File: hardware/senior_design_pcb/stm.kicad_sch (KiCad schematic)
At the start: 46 parts, among them J1 SBH11-PBPC-D05-ST-BK, J2 USB_C_Receptacle_USB2.0_16P, J3 Conn_01x03_Socket, J4 Conn_02x08_Odd_Even, J5 Conn_01x03_Socket, J6 Conn_01x03_Socket, SW1 SW_Push, U1 LD1117S33TR_SOT223, U2 STM32F091RCTx, U3 FT232RL, X1 32.768kHz(12.5pF), X3 8MHz(20pF)

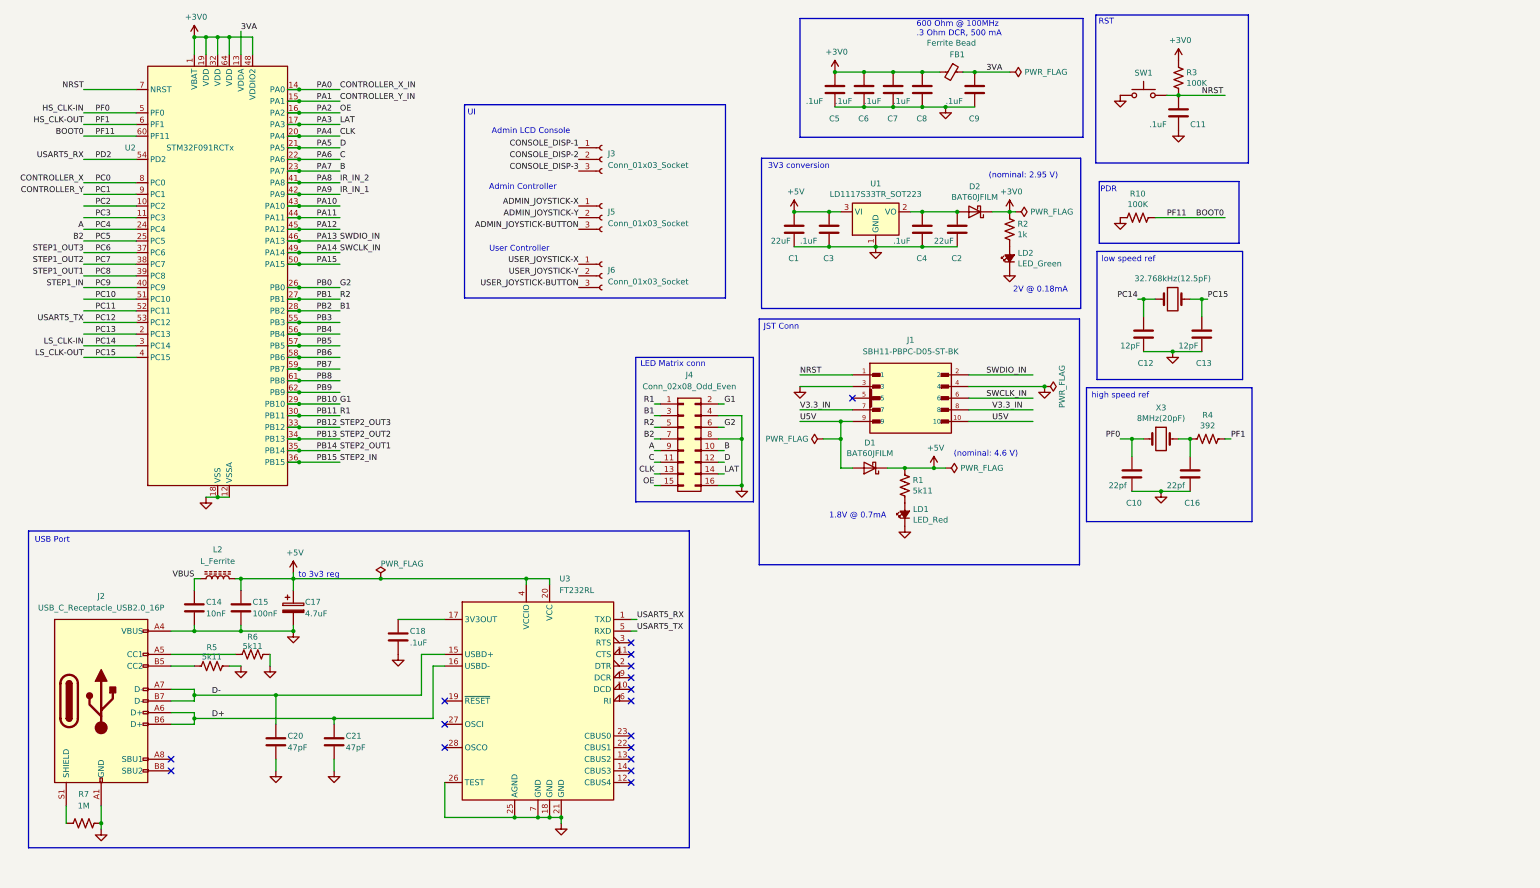
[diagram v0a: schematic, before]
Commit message: small tweaks
added connectors
added shapes
added button
moved shapes
made bigger sheet
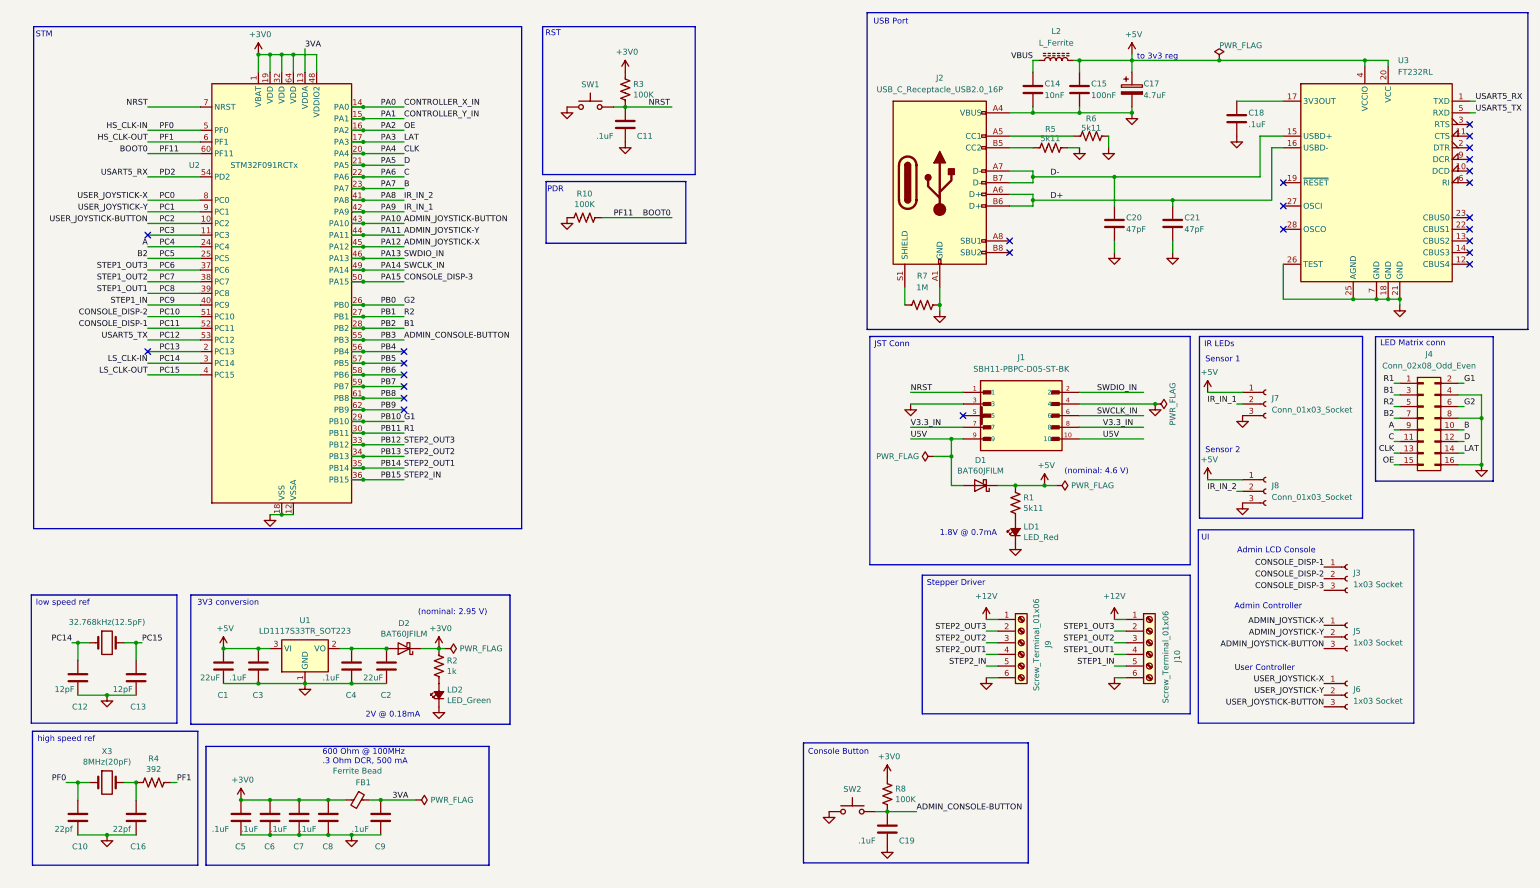
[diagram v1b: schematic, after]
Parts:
- added C19: .1uF, Capacitor_SMD:C_0805_2012Metric_Pad1.15x1.40mm_HandSolder, symbol Device:C
- added J10, J9: Screw_Terminal_01x06, symbol Connector:Screw_Terminal_01x06
- added J7, J8: Conn_01x03_Socket, symbol Connector:Conn_01x03_Socket
- added R8: 100K, Resistor_SMD:R_0805_2012Metric_Pad1.15x1.40mm_HandSolder, symbol Device:R_US
- added SW2: SW_Push, Connector_PinHeader_1.00mm:PinHeader_1x02_P1.00mm_Vertical, symbol Switch:SW_Push
- J3, J5, J6: value Conn_01x03_Socket -> 1x03 Socket
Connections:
- net PA10 is gone; now on net ADMIN_JOYSTICK-BUTTON: U2.43 (PA10)
- net PA11 is gone; now on net ADMIN_JOYSTICK-Y: U2.44 (PA11)
- net PA12 is gone; now on net ADMIN_JOYSTICK-X: U2.45 (PA12)
- net PA15 is gone; now on net CONSOLE_DISP-3: U2.50 (PA15)
- net PC10 is gone; now on net CONSOLE_DISP-2: U2.51 (PC10)
- net PC11 is gone; now on net CONSOLE_DISP-1: U2.52 (PC11)
- net USER_JOYSTICK-BUTTON is gone; now on net PC2: J6.3 (Pin_3)
- net USER_JOYSTICK-X is gone; now on net PC0: J6.1 (Pin_1)
- net USER_JOYSTICK-Y is gone; now on net PC1: J6.2 (Pin_2)
- net +3V0: now also R8.1
- net +5V: now also J7.1 (Pin_1), J8.1 (Pin_1)
- net GND: now also C19.2, J10.6 (Pin_6), J7.3 (Pin_3), J8.3 (Pin_3), J9.6 (Pin_6), SW2.1
- net IR_IN_1: now also J7.2 (Pin_2)
- net IR_IN_2: now also J8.2 (Pin_2)
- net PB12: now also J9.2 (Pin_2)
- net PB13: now also J9.3 (Pin_3)
- net PB14: now also J9.4 (Pin_4)
- net PB15: now also J9.5 (Pin_5)
- net PC6: now also J10.2 (Pin_2)
- net PC7: now also J10.3 (Pin_3)
- net PC8: now also J10.4 (Pin_4)
- net PC9: now also J10.5 (Pin_5)
- net CONTROLLER_X renamed PC0
- net CONTROLLER_Y renamed PC1
- net PB3 renamed ADMIN_CONSOLE-BUTTON
- net ADMIN_CONSOLE-BUTTON: now also C19.1, R8.2, SW2.2
- new net +12V: J10.1 (Pin_1), J9.1 (Pin_1)
- no-connect marks 17 -> 25
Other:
- note added: "Console Button"
- note added: "IR LEDs"
- note added: "STM"
- note added: "Sensor 1"
- note added: "Sensor 2"
- note added: "Stepper Driver"
- moved on the sheet: C1, C10, C11, C12, C13, C14, C15, C16, C17, C18, C2, C20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

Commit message: made it look nice
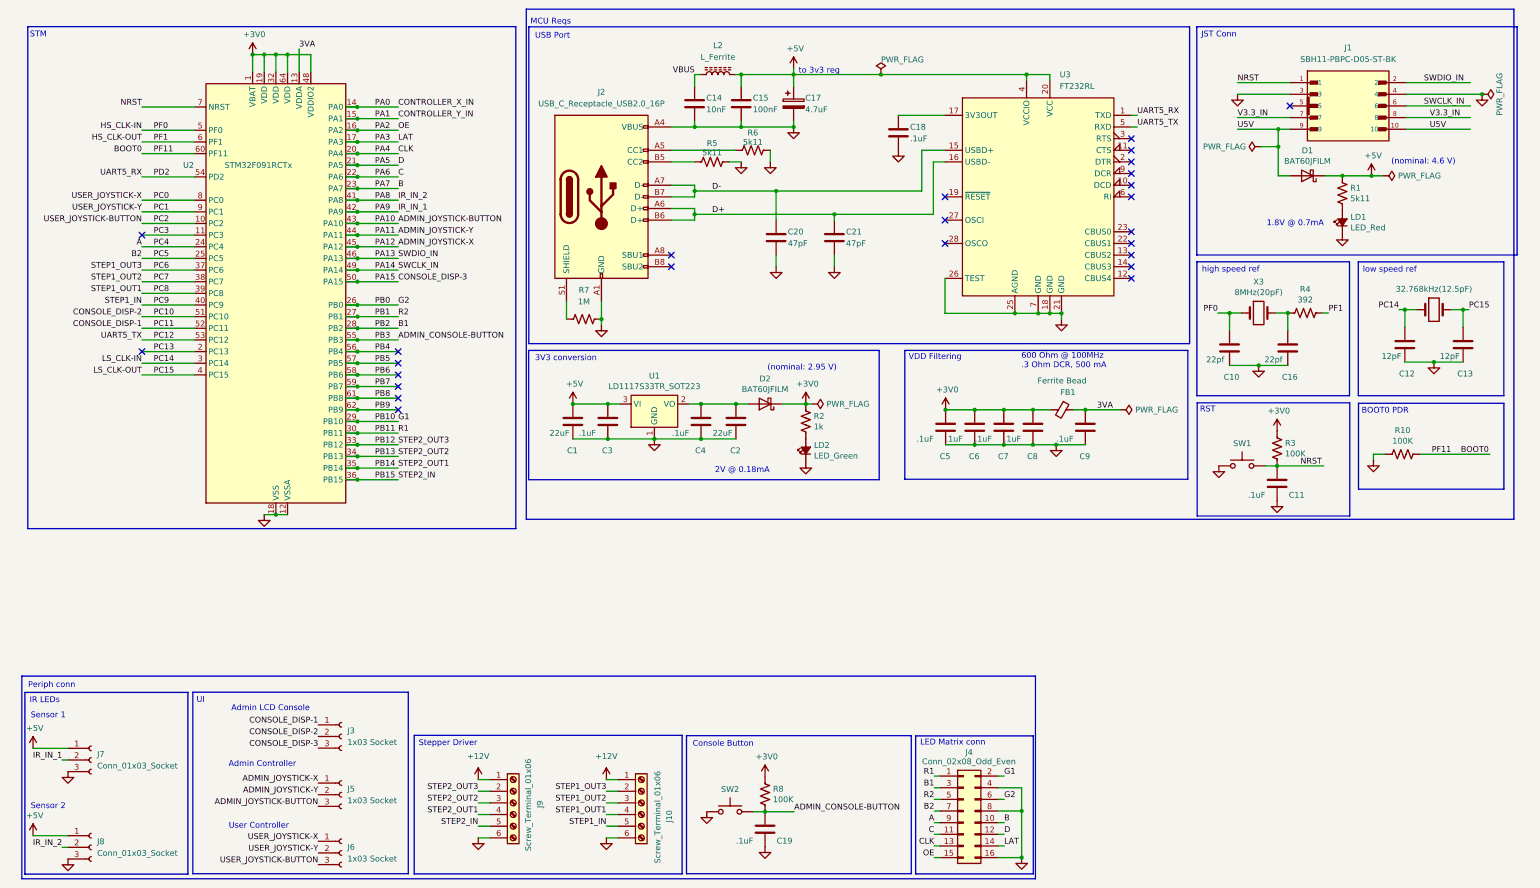
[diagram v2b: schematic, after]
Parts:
- C14, C15, C17, C18, C20, C21: footprint (none) -> Capacitor_SMD:C_0805_2012Metric_Pad1.15x1.40mm_HandSolder
- L2: footprint (none) -> Resistor_SMD:R_0805_2012Metric_Pad1.15x1.40mm_HandSolder
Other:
- note added: "BOOT0 PDR"
- note added: "MCU Reqs"
- note added: "Periph conn"
- note added: "VDD Filtering"
- note removed: "PDR"
- moved on the sheet: C1, C10, C11, C12, C13, C14, C15, C16, C17, C18, C19, C2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
